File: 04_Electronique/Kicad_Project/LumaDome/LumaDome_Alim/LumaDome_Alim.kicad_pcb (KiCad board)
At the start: 4 copper layers, 72.2 x 75 mm, 63 parts, among them J1 USB_C_Receptacle_PowerOnly_6P, J10 Conn_01x04, J3 Conn_01x02, J7 Conn_02x05_Counter_Clockwise, J8 Conn_01x03, J9 Conn_02x03_Counter_Clockwise, Q1 FDS9435A, SW1 SW_SPDT, U1 CYPD3177-24LQ, U3 WE: 173020536, U4 WE: 173010335, U6 ESP32-WROOM-32E, U7 74AHCT125

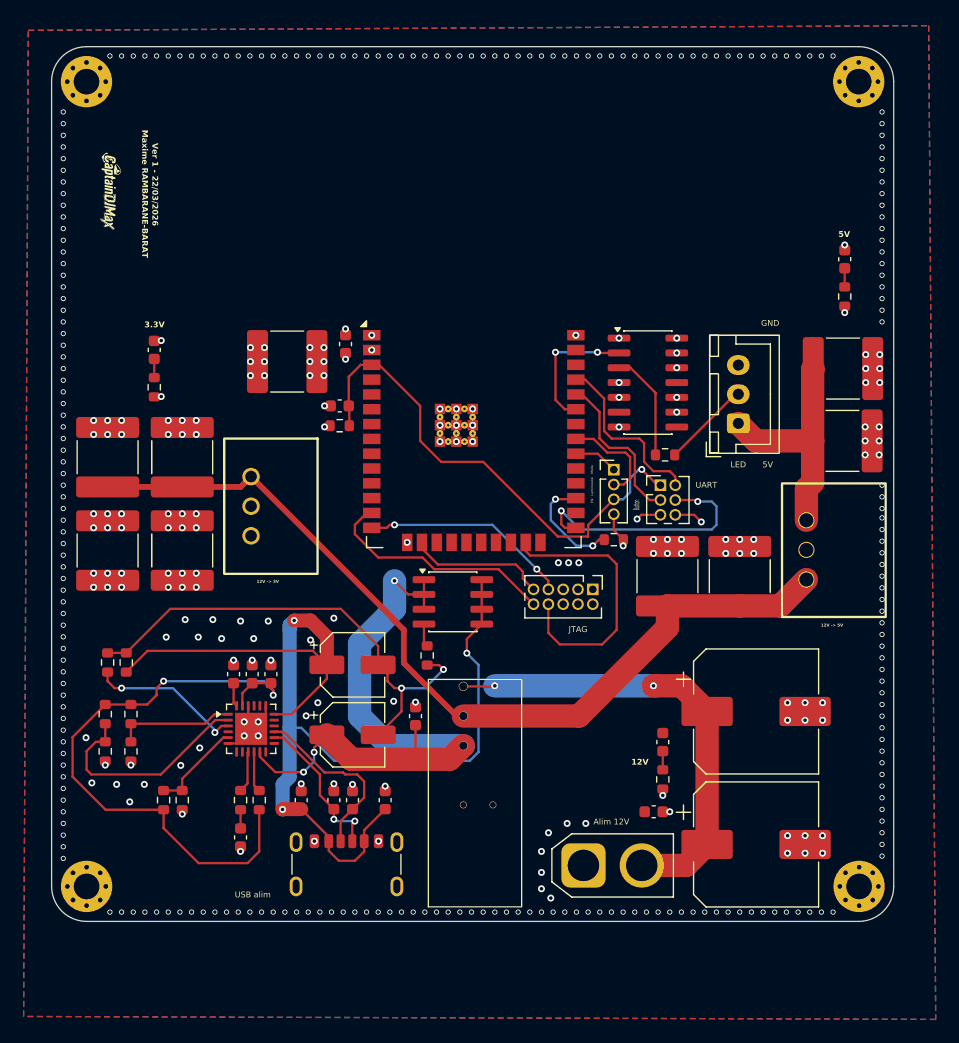
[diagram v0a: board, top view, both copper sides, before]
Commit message: finalisation PCB
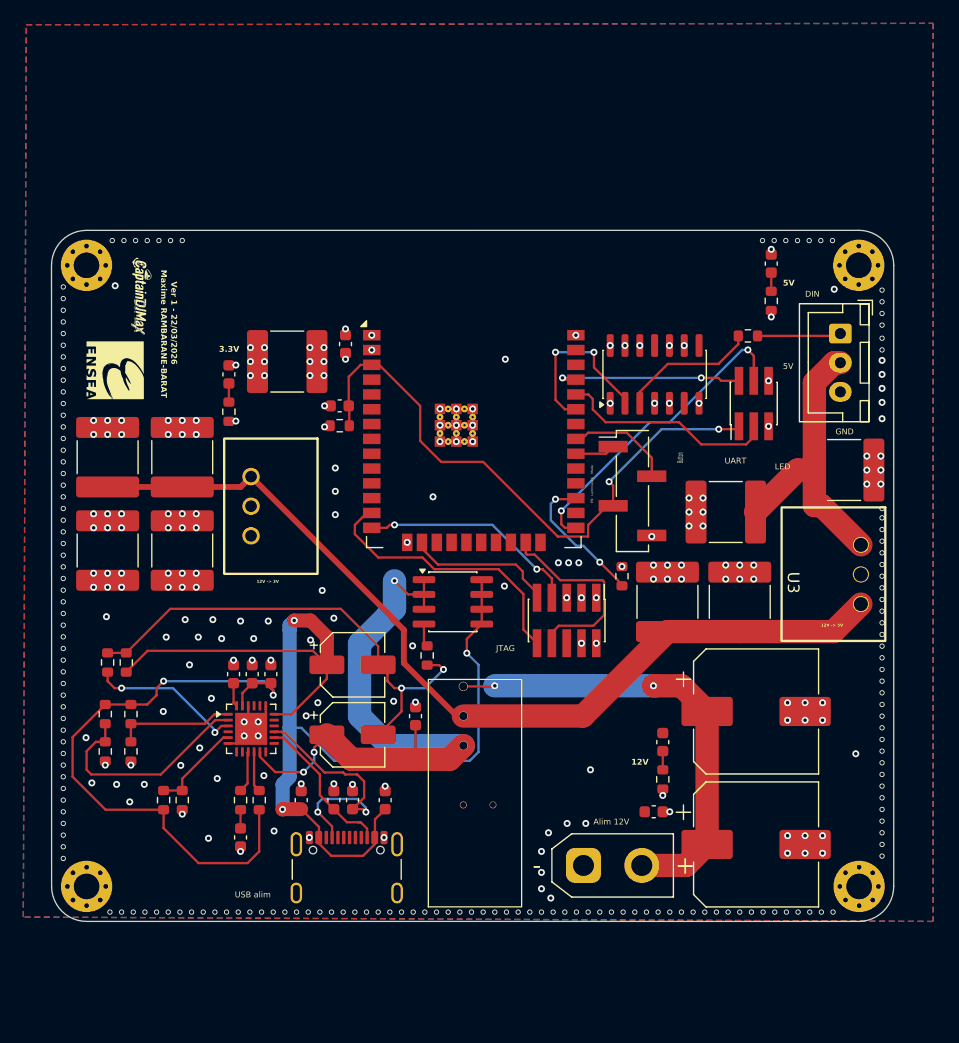
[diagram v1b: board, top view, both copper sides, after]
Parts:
- added G***: LOGO, Logos:logoENSEA, F.Cu at (165.2, 48.8)
- J1: value USB_C_Receptacle_PowerOnly_6P -> USB_C_Receptacle_USB2.0_16P; footprint Connector_USB:USB_C_Receptacle_GCT_USB4125-xx-x-0190_6P_TopMnt_Horizontal -> Connector_USB:USB_C_Receptacle_GCT_USB4105-xx-A_16P_TopMnt_Horizontal
- J10: footprint Connector_PinHeader_1.27mm:PinHeader_1x04_P1.27mm_Vertical -> Connector_PinHeader_2.54mm:PinHeader_1x04_P2.54mm_Vertical_SMD_Pin1Left
- J3: footprint Connector_AMASS:AMASS_XT30U-M_1x02_P5.0mm_Vertical -> Connector_AMASS:AMASS_XT30UPB-F_1x02_P5.0mm_Vertical
- J7: footprint Connector_PinHeader_1.27mm:PinHeader_2x05_P1.27mm_Vertical -> Connector_PinHeader_1.27mm:PinHeader_2x05_P1.27mm_Vertical_SMD
- J9: footprint Connector_PinHeader_1.27mm:PinHeader_2x03_P1.27mm_Vertical -> Connector_PinHeader_1.27mm:PinHeader_2x03_P1.27mm_Vertical_SMD
- moved C22 15.9 mm to (217.6, 60.9), turned to 180 degrees
- moved H1 15.7 mm to (162.8, 39.7)
- moved H2 15.7 mm to (229.0, 39.7)
- moved U3 13.0 mm to (231.3, 60.5), turned to -90 degrees
- moved R1 12.4 mm to (219.5, 45.8)
- moved J8 11.7 mm to (227.4, 45.6), turned to -90 degrees
- moved J9 10.6 mm to (220.0, 51.6), turned to 90 degrees
- moved REF** 9.38 mm to (167.4, 42.0)
- moved D6 6.74 mm to (175.0, 49.1)
- moved R15 6.74 mm to (175.0, 52.3)
- moved D5 6.31 mm to (221.5, 39.6)
- moved R14 6.31 mm to (221.5, 42.8)
- moved J7 3.49 mm to (204.0, 70.2)
- moved R18 3.21 mm to (208.7, 66.4), turned to 90 degrees
- moved C18 2.50 mm to (227.8, 57.3)
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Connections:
- J8 pad 1: +5V -> /ESP 32/DIN
- J8 pad 2: /ESP 32/DIN -> +5V
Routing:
- net /ESP 32/EN: track 43.4 -> 52.1 mm, vias 1 -> 2
- net Net-(J1-CC1): track 15.5 -> 22.0 mm, vias 0 -> 2
- net /ESP 32/ESP_TDO: track 23.9 -> 18.4 mm
- net +5V: track 20.2 -> 25.4 mm
- net /ESP 32/ESP_IO0: track 22.0 -> 27.1 mm
- net +3.3V: track 5.01 -> 0.00 mm, vias 24 -> 26
- net /ESP 32/ESP_RXD: track 13.8 -> 18.7 mm
- net /ESP 32/ESP_TMS: track 20.5 -> 24.0 mm
- net /ESP 32/GPIO_lvl_shfit: track 11.6 -> 14.9 mm
- net Net-(U6-IO16): track 9.46 -> 12.3 mm
- net /Power/SW_Sortie: track 76.4 -> 79.1 mm
- net Net-(R1-Pad1): track 9.34 -> 11.8 mm
- net GND: track 14.0 -> 11.8 mm, vias 379 -> 329
- net /ESP 32/ESP_TXD: track 15.3 -> 16.5 mm, vias 0 -> 2
- net /ESP 32/ESP_TDI: track 18.0 -> 19.1 mm
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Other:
- board size 72.2 x 75 mm -> 72.2 x 59.3 mm
- board text added: "DIN"
